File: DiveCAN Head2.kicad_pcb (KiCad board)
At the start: 4 copper layers, 114.5 x 25 mm, 106 parts, among them J1 C1, J2 C2, J3 C3, J4 AUX, J5 Solenoid, J6 SSC1, J7 CAN, J8 SSC1, J9 SSC1, Q1 DMG1012T, Q2 DMG1012T, Q3 DMG1012T, Q4 DMG1012T, U1 ADS1115IDGS, U2 ADS1115IDGS, U3 NBM7100A, U4 TPS63000, U5 STM32L431RCTx, U6 TCAN33X, Y1 8MHz

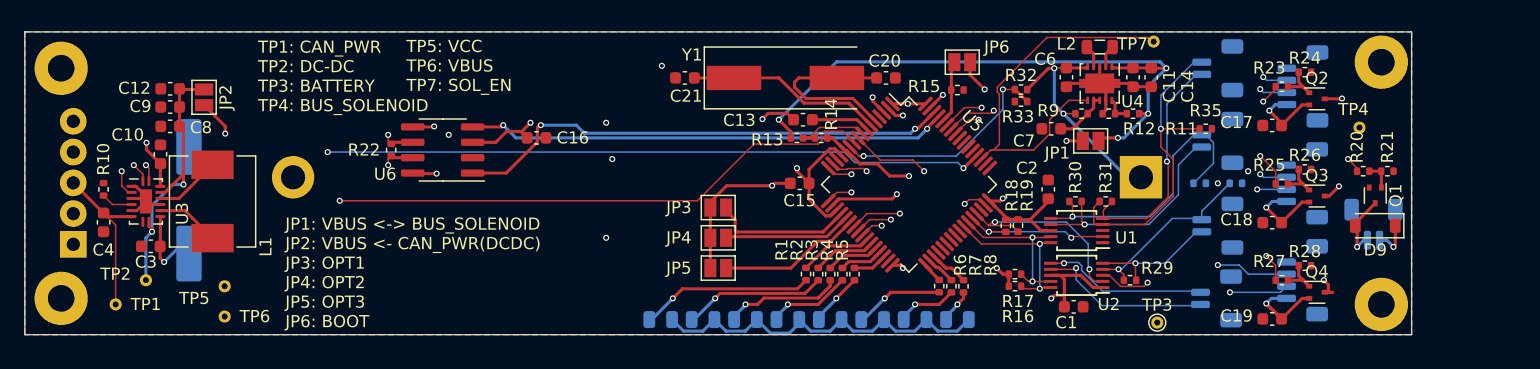
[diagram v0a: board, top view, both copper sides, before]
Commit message: Revision 2.1 HW
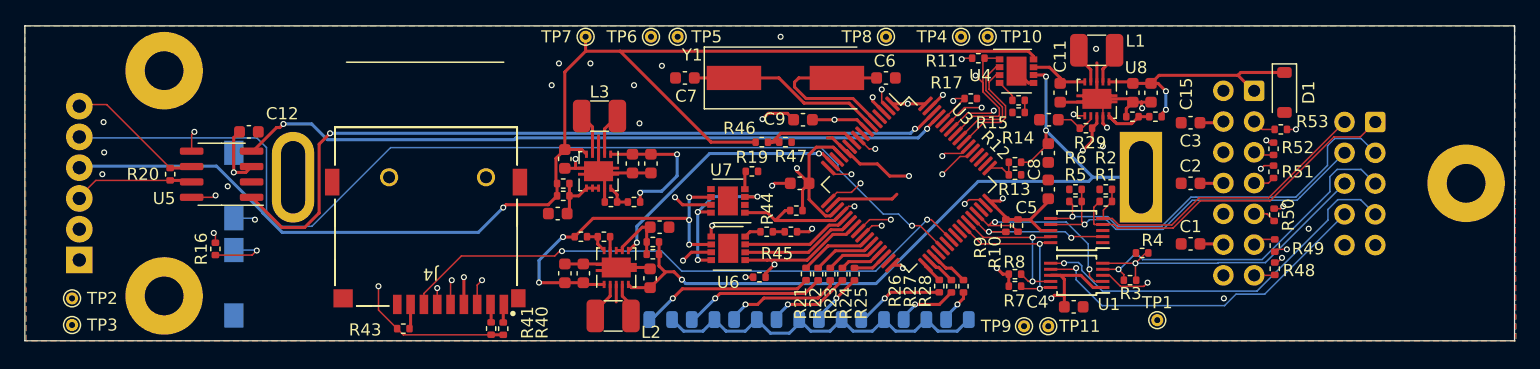
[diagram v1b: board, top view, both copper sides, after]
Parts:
- removed the C10 at (89.7, 82.1)
- removed the C12 at (90.5, 76.7)
- removed the C4 at (85.0, 87.7)
- removed the C5 at (92.0, 85.9)
- removed the C6 at (164.5, 75.8)
- removed the C7 at (163.2, 80.0)
- removed the C9 at (90.5, 78.2)
- removed H3: MountingHole_Pad, MountingHole:MountingHole_2.2mm_M2_Pad
- removed J5: Solenoid, Connector_JST:JST_SH_BM02B-SRSS-TB_1x02-1MP_P1.00mm_Vertical
- removed J6, J8, J9: SSC1, Connector_JST:JST_SH_BM04B-SRSS-TB_1x04-1MP_P1.00mm_Vertical
- removed J7: CAN, TerminalBlock_Phoenix:TerminalBlock_Phoenix_MPT-0,5-5-2.54_1x05_P2.54mm_Horizontal
- removed JP1, JP2, JP3, JP4, JP5, JP6: ~, Jumper:SolderJumper-2_P1.3mm_Open_Pad1.0x1.5mm
- removed Q1, Q2, Q3, Q4: DMG1012T, Package_TO_SOT_SMD:SOT-523
- removed the R10 at (85.0, 85.0)
- removed the R20 at (189.0, 83.5)
- removed the R21 at (191.0, 83.5)
- removed the R23 at (182.3, 76.5)
- removed the R24 at (184.2, 75.3)
- removed the R25 at (182.3, 84.5)
- removed the R26 at (184.2, 83.3)
- removed the R27 at (182.3, 92.5)
- removed the R28 at (184.2, 91.3)
- removed the R9 at (165.8, 78.8)
- removed the TP2 at (88.5, 92.5)
- removed the TP3 at (172.0, 96.0)
- removed the TP4 at (188.7, 79.9)
- removed the U3 at (88.5, 86.0)
- added C1: 100n, Capacitor_SMD:C_0603_1608Metric, F.Cu at (174.8, 89.5)
- added C13: 100n, Capacitor_SMD:C_0603_1608Metric, F.Cu at (163.1, 79.2)
- added C15: 10u, Capacitor_SMD:C_0603_1608Metric, F.Cu at (171.5, 77.0)
- added C16: 100n, Capacitor_SMD:C_0603_1608Metric, F.Cu at (130.9, 88.1)
- added C2: 100n, Capacitor_SMD:C_0603_1608Metric, F.Cu at (174.8, 84.5)
- added C20: 10u, Capacitor_SMD:C_0603_1608Metric, F.Cu at (128.7, 82.9)
- added C21: 10u, Capacitor_SMD:C_0603_1608Metric, F.Cu at (130.2, 82.9)
- added C22: 10u, Capacitor_SMD:C_0603_1608Metric, F.Cu at (130.1, 92.3)
- added C23: 10u, Capacitor_SMD:C_0603_1608Metric, F.Cu at (123.1, 82.5)
- added L3: 2.2u, Library:L_4x4, F.Cu at (126.0, 79.0)
- added R15: 200, Resistor_SMD:R_0402_1005Metric, F.Cu at (160.6, 77.7)
- added R16: 10k, Resistor_SMD:R_0402_1005Metric, F.Cu at (94.2, 89.9)
- added R18: 10k, Resistor_SMD:R_0402_1005Metric, F.Cu at (142.2, 86.8)
- added R19: 800, Resistor_SMD:R_0402_1005Metric, F.Cu at (138.5, 83.5)
- added R2: 200, Resistor_SMD:R_0402_1005Metric, F.Cu at (167.8, 85.0)
- added R29: 200, Resistor_SMD:R_0402_1005Metric, F.Cu at (166.1, 79.9)
- added R30: 1M, Resistor_SMD:R_0402_1005Metric, F.Cu at (171.8, 79.0)
- added R31: 100k, Resistor_SMD:R_0402_1005Metric, F.Cu at (169.9, 79.0)
- added R37: 200, Resistor_SMD:R_0402_1005Metric, F.Cu at (123.0, 85.5)
- added R38: 1M, Resistor_SMD:R_0402_1005Metric, F.Cu at (128.8, 86.0)
- added R39: 178k, Resistor_SMD:R_0402_1005Metric, F.Cu at (126.9, 86.0)
- added R4: 200, Resistor_SMD:R_0402_1005Metric, F.Cu at (170.8, 90.2)
- added R40: 10k, Resistor_SMD:R_0402_1005Metric, F.Cu at (118.0, 96.5)
- added R41: 10k, Resistor_SMD:R_0402_1005Metric, F.Cu at (117.0, 96.5)
- added R42: 200, Resistor_SMD:R_0402_1005Metric, F.Cu at (141.8, 88.5)
- added R43: 10k, Resistor_SMD:R_0402_1005Metric, F.Cu at (109.8, 96.5)
- added R44: 200, Resistor_SMD:R_0402_1005Metric, F.Cu at (139.8, 88.5)
- added R45: 10k, Resistor_SMD:R_0402_1005Metric, F.Cu at (139.2, 92.2)
- added R46: 10k, Resistor_SMD:R_0402_1005Metric, F.Cu at (139.3, 81.1)
- added R47: 10k, Resistor_SMD:R_0402_1005Metric, F.Cu at (141.3, 81.1)
- added R48: 800, Resistor_SMD:R_0402_1005Metric, F.Cu at (181.7, 91.5)
- added R49: 800, Resistor_SMD:R_0402_1005Metric, F.Cu at (181.7, 89.6)
- added R50: 800, Resistor_SMD:R_0402_1005Metric, F.Cu at (181.7, 87.1)
- added R51: 800, Resistor_SMD:R_0402_1005Metric, F.Cu at (181.6, 83.5)
- added R52: 800, Resistor_SMD:R_0402_1005Metric, F.Cu at (181.6, 81.7)
- added R53: 800, Resistor_SMD:R_0402_1005Metric, F.Cu at (182.2, 80.0)
- added R6: 200, Resistor_SMD:R_0402_1005Metric, F.Cu at (165.2, 85.0)
- added SW1: RST, Button_Switch_SMD:SW_SPST_EVQPE1, B.Cu at (95.8, 92.7)
- added SW2: RST, Button_Switch_SMD:SW_SPST_EVQPE1, B.Cu at (95.8, 84.7)
- added TP10: SOL_STAT, TestPoint:TestPoint_THTPad_D1.0mm_Drill0.5mm, F.Cu at (158.0, 72.4)
- added TP11: VCC_STAT, TestPoint:TestPoint_THTPad_D1.0mm_Drill0.5mm, F.Cu at (163.0, 96.3)
- added TP5: BAT_REG, TestPoint:TestPoint_THTPad_D1.0mm_Drill0.5mm, F.Cu at (132.4, 72.4)
- added TP6: CAN_REG, TestPoint:TestPoint_THTPad_D1.0mm_Drill0.5mm, F.Cu at (130.2, 72.4)
- added TP7: CAN_PWR, TestPoint:TestPoint_THTPad_D1.0mm_Drill0.5mm, F.Cu at (124.8, 72.4)
- added TP8: BAT_EN, TestPoint:TestPoint_THTPad_D1.0mm_Drill0.5mm, F.Cu at (149.6, 72.4)
- added TP9: BUS_STAT, TestPoint:TestPoint_THTPad_D1.0mm_Drill0.5mm, F.Cu at (161.0, 96.3)
- added U10: TPS63000, Package_SON:Texas_DRC0010J, F.Cu at (125.9, 83.5)
- added U6: TPS2115, Library:VSON-8_3.3x3.3mm_P0.65mm_NexFET, F.Cu at (136.6, 89.9)
- added U7: TPS2115, Library:VSON-8_3.3x3.3mm_P0.65mm_NexFET, F.Cu at (136.6, 86.0)
- added U8: TPS63000, Package_SON:Texas_DRC0010J, F.Cu at (167.0, 77.5)
- added U9: TPS63000, Package_SON:Texas_DRC0010J, F.Cu at (127.3, 91.5)
- C17, C18: value 100n -> 10u
- H1, H2, H4: footprint MountingHole:MountingHole_2.2mm_M2_Pad -> MountingHole:MountingHole_3.2mm_M3_Pad
- J1: value C1 -> Analog Connection; footprint Connector_JST:JST_SH_BM02B-SRSS-TB_1x02-1MP_P1.00mm_Vertical -> Connector_IDC:IDC-Header_2x05_P2.54mm_Vertical
- J2: value C2 -> Digital Connection; footprint Connector_JST:JST_SH_BM02B-SRSS-TB_1x02-1MP_P1.00mm_Vertical -> Connector_IDC:IDC-Header_2x07_P2.54mm_Vertical
- J3: value C3 -> Conn_01x06_Pin; footprint Connector_JST:JST_SH_BM02B-SRSS-TB_1x02-1MP_P1.00mm_Vertical -> TerminalBlock_Phoenix:TerminalBlock_Phoenix_MPT-0,5-6-2.54_1x06_P2.54mm_Horizontal
- J4: value AUX -> Micro_SD_Card; footprint Connector_JST:JST_SH_BM02B-SRSS-TB_1x02-1MP_P1.00mm_Vertical -> Library:CONN9_0185-02_GSW; moved to F.Cu
- L1: value 15u -> 2.2u; footprint Inductor_SMD:L_Sunlord_MWSA0604S -> Library:L_4x4
- L2: footprint Inductor_SMD:L_0805_2012Metric -> Library:L_4x4
- R11: value 1M -> 10k
- R12: value 178k -> 10k
- R14, R32, R33: value 10k -> 200
- R34: value 200 -> 1M; moved to F.Cu
- R35: value 200 -> 178k
- R36: moved to F.Cu
- TP1: value CAN_PWR -> BATTERY; moved to F.Cu
- TP2: renamed from TP5; moved to F.Cu
- TP3: renamed from TP6; moved to F.Cu
- TP4: renamed from TP7; moved to F.Cu
- U4: value TPS63000 -> TPS2115; footprint Package_SON:Texas_DRC0010J -> Library:VSON-8_3.3x3.3mm_P0.65mm_NexFET
- moved J3 94.0 mm to (83.0, 90.8)
- moved C3 86.5 mm to (174.8, 79.5), turned to 0 degrees
- moved TP1 86.0 mm to (172.0, 95.8), turned to 0 degrees
- moved L1 74.1 mm to (167.0, 73.5), turned to 180 degrees
- moved C8 72.5 mm to (163.0, 82.0), turned to 90 degrees
- moved C19 59.6 mm to (122.5, 87.0), turned to 0 degrees
- moved J4 58.8 mm to (118.1, 94.5), turned to 180 degrees
- moved C18 58.5 mm to (123.1, 91.9), turned to 90 degrees
- moved C17 58.2 mm to (124.6, 91.9), turned to 90 degrees
- moved R36 55.5 mm to (123.0, 84.5), turned to 180 degrees
- moved R34 51.3 mm to (124.4, 88.9)
- moved R35 50.5 mm to (126.3, 88.9)
- moved L2 45.9 mm to (127.1, 95.4), turned to 0 degrees
- moved R32 33.3 mm to (130.4, 90.4)
- moved R33 32.5 mm to (130.4, 89.3)
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- renumbered C15 to C10, C16 to C12, C1 to C4, C2 to C5, C20 to C6, C21 to C7, C13 to C9, D9 to D1, D1 to D2, D2 to D3, D3 to D4, D4 to D5, D5 to D6, D6 to D7, D7 to D8, D8 to D9, R31 to R1, R19 to R10, R15 to R17, R22 to R20, R1 to R21, R2 to R22, R3 to R23, R4 to R24, R5 to R25, R6 to R26, R7 to R27, R8 to R28, R29 to R3, R30 to R5, R16 to R7, R17 to R8, R18 to R9, U2 to U1, U1 to U2, U5 to U3, U6 to U5
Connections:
- net Net-(U5-NRST) renamed /RST
- C11 pad 1: /BUS_SOLENOID -> GNDREF
- C11 pad 2: GNDREF -> /Solenoid Driver/IN
- C14 pad 1: /BUS_SOLENOID -> /SOL_OUT
- C17 pad 1: Net-(J6-Pin_1) -> /BATTERY_REGULATED
- C18 pad 1: Net-(J8-Pin_1) -> /BATTERY_REGULATED
- C19 pad 1: Net-(J9-Pin_1) -> GNDREF
- C19 pad 2: GNDREF -> Net-(U10-EN)
- C3 pad 1: Net-(U3-CAP) -> GNDREF
- C3 pad 2: GNDREF -> VBUS
- C8 pad 2: /CAN Power Converter/OUT_BOOST -> /BATTERY
- D1 pad 1: /BUS_SOLENOID -> /SOL_OUT
- D1 pad 2: Net-(D9-A) (its old number) -> GNDREF
- J1 pad 1: Net-(J1-Pin_1) -> /C1+
- J1 pad 2: Net-(J1-Pin_2) -> /C1-
- J2 pad 1: Net-(J2-Pin_1) -> /SOL_OUT
- J2 pad 2: Net-(J2-Pin_2) -> GNDREF
- J3 pad 1: Net-(J3-Pin_1) -> VBUS
- J3 pad 2: Net-(J3-Pin_2) -> GNDREF
- J4 pad 1: Net-(J4-Pin_1) -> Net-(J4-DAT2)
- J4 pad 2: Net-(J4-Pin_2) -> Net-(J4-DAT3/CD)
- L2 pad 1: Net-(U4-L2) -> Net-(U9-L2)
- L2 pad 2: Net-(U4-L1) -> Net-(U9-L1)
- R1 pad 1: Net-(J1-Pin_2) -> /C1+
- R1 pad 2: Net-(J1-Pin_1) -> /C1-
- R11 pad 1: /BUS_SOLENOID -> VCC
- R11 pad 2: Net-(U4-FB) -> /SOL_STAT
- R12 pad 1: Net-(U4-FB) -> Net-(U3-PA14)
- R12 pad 2: GNDREF -> /BATTERY
- R13 pad 1: Net-(U5-PC0) -> GNDREF
- R13 pad 2: /BUS_SOLENOID -> Net-(U3-PA14)
- R14 pad 2: Net-(U5-PC0) -> Net-(R14-Pad2)
- R20 pad 1: Net-(J7-Pin_2) -> Net-(J3-Pin_3)
- R20 pad 2: Net-(J7-Pin_5) -> Net-(J3-Pin_6)
- R3 pad 1: Net-(J3-Pin_2) -> /C3+
- R3 pad 2: Net-(J3-Pin_1) -> /C3-
- R32 pad 1: Net-(U5-PC3) -> Net-(U9-PS/SYNC)
- R33 pad 1: GNDREF -> Net-(U9-PS/SYNC)
- R33 pad 2: Net-(U5-PC3) -> /BATTERY
- R34 pad 1: Net-(J2-Pin_2) -> /BATTERY_REGULATED
- R34 pad 2: GNDREF -> Net-(U9-FB)
- R35 pad 1: Net-(J1-Pin_2) -> Net-(U9-FB)
- R36 pad 1: Net-(J3-Pin_2) -> Net-(U10-EN)
- R36 pad 2: GNDREF -> /CAN_PWR
- R5 pad 1: Net-(J2-Pin_2) -> /C2+
- R5 pad 2: Net-(J2-Pin_1) -> /C2-
- TP1 pad 1: /CAN_PWR -> /BATTERY
- TP4 pad 1: /CONVERTER_EN -> /SOLENOID
- U1 pad 4: Net-(J3-Pin_2) -> /C3+
- U1 pad 5: Net-(J3-Pin_1) -> /C3-
- U1 pad 6: Net-(J4-Pin_2) -> /AUX+
- U1 pad 7: Net-(J4-Pin_1) -> /AUX-
- U2 pad 4: Net-(J1-Pin_2) -> /C1+
- U2 pad 5: Net-(J1-Pin_1) -> /C1-
- U2 pad 6: Net-(J2-Pin_2) -> /C2+
- U2 pad 7: Net-(J2-Pin_1) -> /C2-
- U3 pad 10: /PWR_RDY -> Net-(U3-PC2)
- U3 pad 11: Net-(U5-PC3) -> unconnected-(U3-PC3-Pad11)
- U3 pad 15: /SSC2_EN -> /BATTERY_EN
- U3 pad 20: Net-(JP3-A) -> /VCC_STAT
- U3 pad 21: Net-(JP4-A) -> /BUS_SEL2
- U3 pad 22: Net-(JP5-A) -> /BUS_SEL1
- U3 pad 23: /SSC3_EN -> /BUS_STAT
- U3 pad 37: unconnected-(U5-PC6-Pad37) -> /~{CAN_EN}
- U3 pad 39: unconnected-(U5-PC8-Pad39) -> /SD_DAT0
- U3 pad 49: unconnected-(U5-PA14-Pad49) -> Net-(U3-PA14)
- U3 pad 51: /CONVERTER_EN -> unconnected-(U3-PC10-Pad51)
- U3 pad 52: /~{CAN_EN} -> unconnected-(U3-PC11-Pad52)
- U3 pad 53: unconnected-(U5-PC12-Pad53) -> /SD_CLK
- U3 pad 54: unconnected-(U5-PD2-Pad54) -> /SD_CMD
- U3 pad 55: unconnected-(U5-PB3-Pad55) -> /SOL_SEL2
- U3 pad 56: unconnected-(U5-PB4-Pad56) -> /SOL_SEL1
- U3 pad 57: /SSC1_EN -> /SOL_STAT
- U3 pad 8: Net-(U5-PC0) -> unconnected-(U3-PC0-Pad8)
- U4 pad 1: /BUS_SOLENOID -> /SOL_STAT
- U4 pad 2: Net-(U4-L2) -> /SOL_SEL1
- U4 pad 3: GNDREF -> /SOL_SEL2
- U4 pad 4: Net-(U4-L1) -> Net-(U4-I_LIM)
- U4 pad 5: /BATTERY -> GNDREF
- U4 pad 6: /CONVERTER_EN -> /BATTERY
- U4 pad 7: Net-(U4-PS/SYNC) -> /Solenoid Driver/IN
- U4 pad 8: Net-(U4-PS/SYNC) -> /CAN_PWR
- U5 pad 6: Net-(J7-Pin_5) -> Net-(J3-Pin_6)
- U5 pad 7: Net-(J7-Pin_2) -> Net-(J3-Pin_3)
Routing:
- net /CAN_PWR: track 13.9 -> 110.7 mm, vias 0 -> 1
- net /BUS_SOLENOID: track 83.1 -> 0.00 mm, vias 5 -> 0
- net /SDA: track 93.9 -> 13.7 mm, vias 3 -> 2
- net /SCL: track 93.9 -> 14.2 mm, vias 3 -> 2
- net /PWR_RDY: track 67.6 -> 0.00 mm, vias 2 -> 0
- net /BOOT: track 4.95 -> 67.6 mm, vias 0 -> 2
- net /RST: track 4.83 -> 62.9 mm, vias 0 -> 2
- net /SD_CMD: track 0.00 -> 49.2 mm, vias 0 -> 2
- net /SD_DAT0: track 0.00 -> 49.0 mm, vias 0 -> 2
- net /SD_CLK: track 0.00 -> 48.8 mm, vias 0 -> 2
- net /CAN_REGULATED: track 0.00 -> 46.7 mm, vias 0 -> 5
- net /BATTERY: track 30.8 -> 74.9 mm, vias 2 -> 3
- net /BATTERY_REGULATED: track 0.00 -> 42.5 mm, vias 0 -> 5
- net /SSC2_EN: track 40.4 -> 0.00 mm, vias 2 -> 0
- net /SSC3_EN: track 39.3 -> 0.00 mm, vias 2 -> 0
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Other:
- board size 114.5 x 25 mm -> 123 x 26 mm
- board text added: "1+ 2+ 3+ A+ V"
- board text added: "1- 2- 3- A- G"
- board text added: "7...0"
- board text added: "BOOT RESET"
- board text added: "CAN_L ENABLE CAN_PWR CAN_H GND VBUS"
- board text added: "DIVE CAN CONTROLLER 2.1"
- board text added: "G V G V G V G"
- board text added: "SOL TX1 RX1 TX2 RX2 TX3 RX3"
- board text added: "TP10"
- board text added: "TP11 TP9"
- board text added: "TP8"
- board text removed: "AUX"
- board text removed: "C1"
- board text removed: "C2"
- board text removed: "C3"
- board text removed: "CAN_L ENABLE VCC CAN_H GND"
- board text removed: "DIVE CAN CONTROLLER 2.0"
- board text removed: "JP1: VBUS <-> BUS_SOLENOID JP2: VBUS <- CAN_PWR(DCDC) JP3: OPT1 JP4: OPT2 JP5: OPT3 JP6: BOOT"
- board text removed: "SOLENOID MAX:0.5A"
- board text removed: "SSC1"
- board text removed: "SSC2"
- board text removed: "SSC3"
- board text removed: "TP1: CAN_PWR TP2: DC-DC TP3: BATTERY TP4: BUS_SOLENOID"
- board text removed: "TP5: VCC TP6: VBUS TP7: SOL_EN"
